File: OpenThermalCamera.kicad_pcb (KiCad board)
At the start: 2 copper layers, 26 x 20 mm, 18 parts, among them J1 Conn_ARM_JTAG_SWD_10, J2 USB_CONN, SW1 PB_Bootloader, U1 MLX90640, U2 TPS793333-EP, U3 STM32F042F6Px, U4 NUP2202

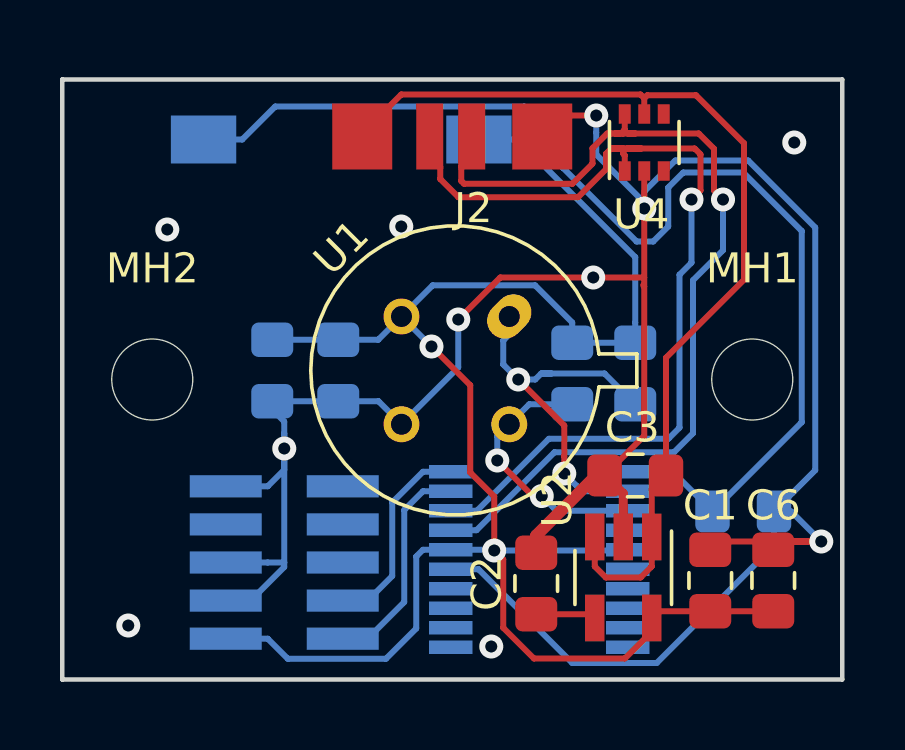
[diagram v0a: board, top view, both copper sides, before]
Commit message: Rev2
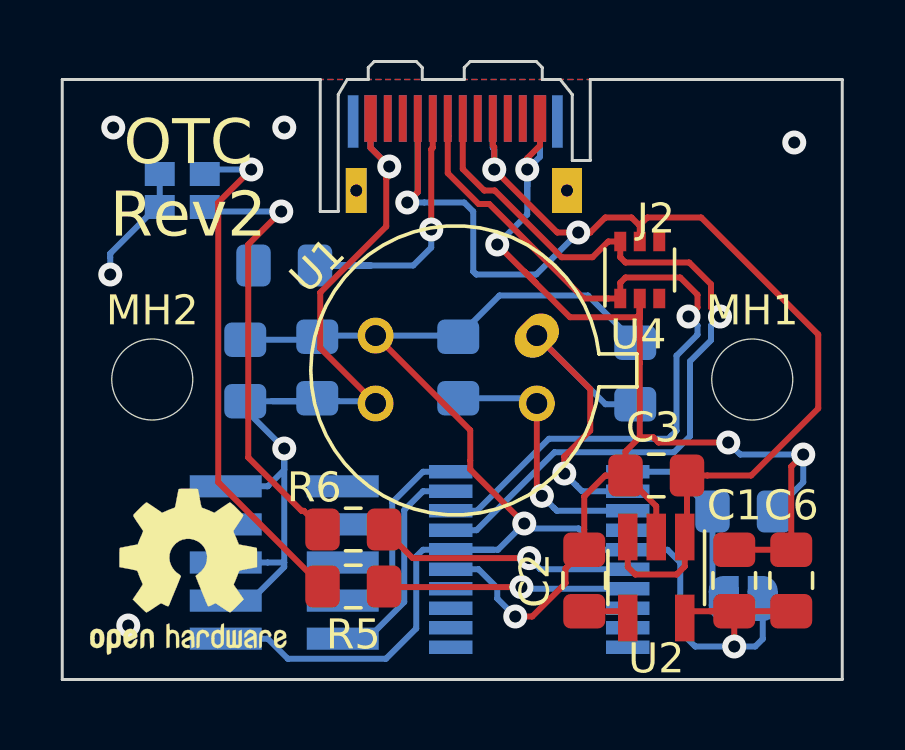
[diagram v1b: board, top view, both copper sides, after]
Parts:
- added D1: LED_Dual_ACAC, LED_SMD:LED_Cree-PLCC4_2x2mm_CW, B.Cu at (31.0, 30.7)
- added G1: , Symbol:OSHW-Logo2_7.3x6mm_SilkScreen, F.Cu at (31.2, 43.4)
- added R4: 5k1, Resistor_SMD:R_0805_2012Metric_Pad1.15x1.40mm_HandSolder, B.Cu at (34.4, 33.2)
- added R5: 10R, Resistor_SMD:R_0805_2012Metric_Pad1.15x1.40mm_HandSolder, F.Cu at (36.7, 43.9)
- added R6: 130R, Resistor_SMD:R_0805_2012Metric_Pad1.15x1.40mm_HandSolder, F.Cu at (36.7, 42.0)
- J2: value USB_CONN -> DX07P024AJ1R1500; footprint usb_b2b_connector:usb_b2b_connector -> lib_fp:DX07P024AJ1R1500
- R2, R3: value 2k2 -> 4k7
- SW1: footprint Button_Switch_SMD:SW_SPST_FSMSM -> Jumper:SolderJumper-2_P1.3mm_Open_RoundedPad1.0x1.5mm
- U1: footprint Package_TO_SOT_THT:TO-39-4_Window -> lib_fp:MLX90640
- moved SW1 20.3 mm to (49.7, 44.3)
- moved J2 4.70 mm to (40.4, 29.5), turned to 180 degrees
- moved U4 4.25 mm to (46.2, 33.4)
- moved R3 3.81 mm to (40.2, 36.6)
- moved C2 1.60 mm to (44.4, 43.7)
- moved U2 1.10 mm to (46.8, 43.6)
- moved C5 0.90 mm to (33.1, 36.7)
- moved C1 0.80 mm to (49.4, 43.7)
- moved C4 0.71 mm to (35.5, 36.6)
- moved C3 0.70 mm to (46.8, 40.2)
- moved C6 0.60 mm to (51.3, 43.7)
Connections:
- U3 pad 17: /USB_P -> /USB_N
- U3 pad 18: /USB_N -> /USB_P
- U3 pad 6: Net-(U3-Pad6) -> /BLUE_LED
- U3 pad 7: Net-(U3-Pad7) -> /RED_LED
- U4 pad 1: /USB_N -> /USB_P
- U4 pad 6: /USB_P -> /USB_N
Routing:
- net /BOOT0: track 39.2 -> 6.43 mm
- net Net-(D1-Pad1): track 0.00 -> 17.4 mm, vias 0 -> 1
- net Net-(D1-Pad4): track 0.00 -> 14.7 mm, vias 0 -> 1
- net +5V: track 33.2 -> 46.0 mm, vias 0 -> 3
- net Net-(J2-PadA5): track 0.00 -> 10.3 mm, vias 0 -> 1
- net /BLUE_LED: track 0.00 -> 8.67 mm, vias 0 -> 1
- net /RED_LED: track 0.00 -> 8.16 mm, vias 0 -> 1
- net GND: track 91.9 -> 84.6 mm, vias 11 -> 12
- net +3V3: track 62.5 -> 56.2 mm
- net /USB_P: track 32.5 -> 26.5 mm
- net /USB_N: track 31.4 -> 27.9 mm
- net /I2C_SDA: track 13.3 -> 12.3 mm, vias 2 -> 1
- net /I2C_SCL: track 8.79 -> 9.21 mm, vias 2 -> 1
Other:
- board size 26 x 20 mm -> 26 x 20.6 mm
- board text added: "OTC Rev2"
